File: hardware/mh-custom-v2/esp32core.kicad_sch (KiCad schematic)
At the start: 1 part, among them U1 ESP32-DEVKITC-32D

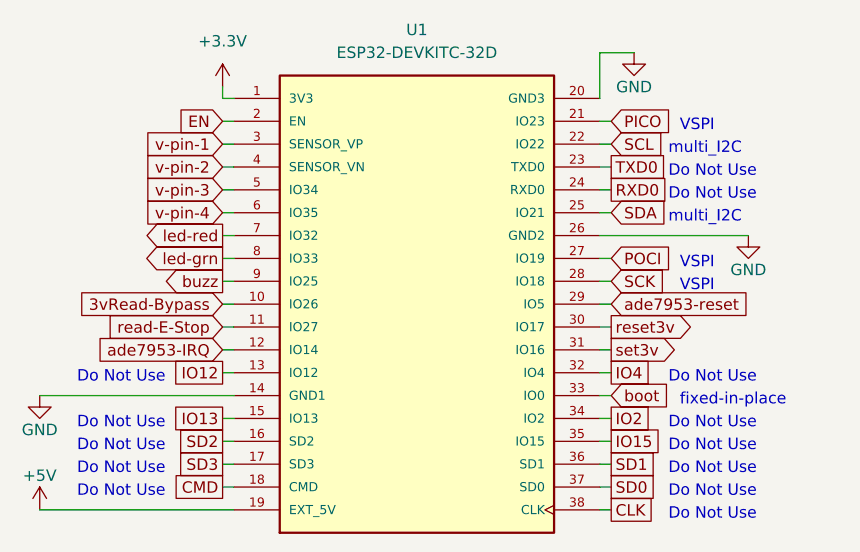
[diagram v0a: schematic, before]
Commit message: laptop back, coordinating efforts
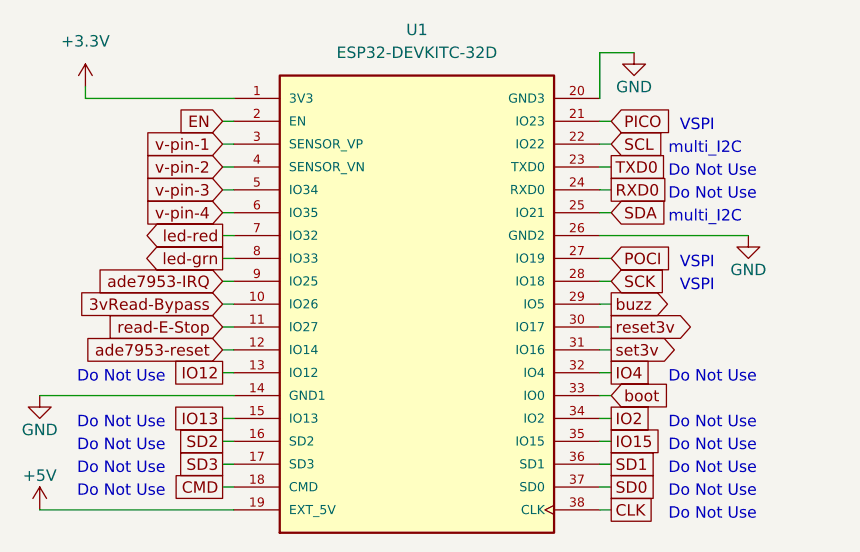
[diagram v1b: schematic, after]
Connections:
- net ade7953-IRQ: now also U1.9 (IO25); no longer U1.12 (IO14)
- net ade7953-reset: now also U1.12 (IO14); no longer U1.29 (IO5)
- net buzz: now also U1.29 (IO5); no longer U1.9 (IO25)
- net +3V3 renamed +3.3V
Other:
- note removed: "fixed-in-place"
